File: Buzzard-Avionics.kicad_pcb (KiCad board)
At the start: 2 copper layers, 30 x 115.5 mm, 6 parts, among them J4 Conn_01x02_Socket, SW1 SW_SPDT

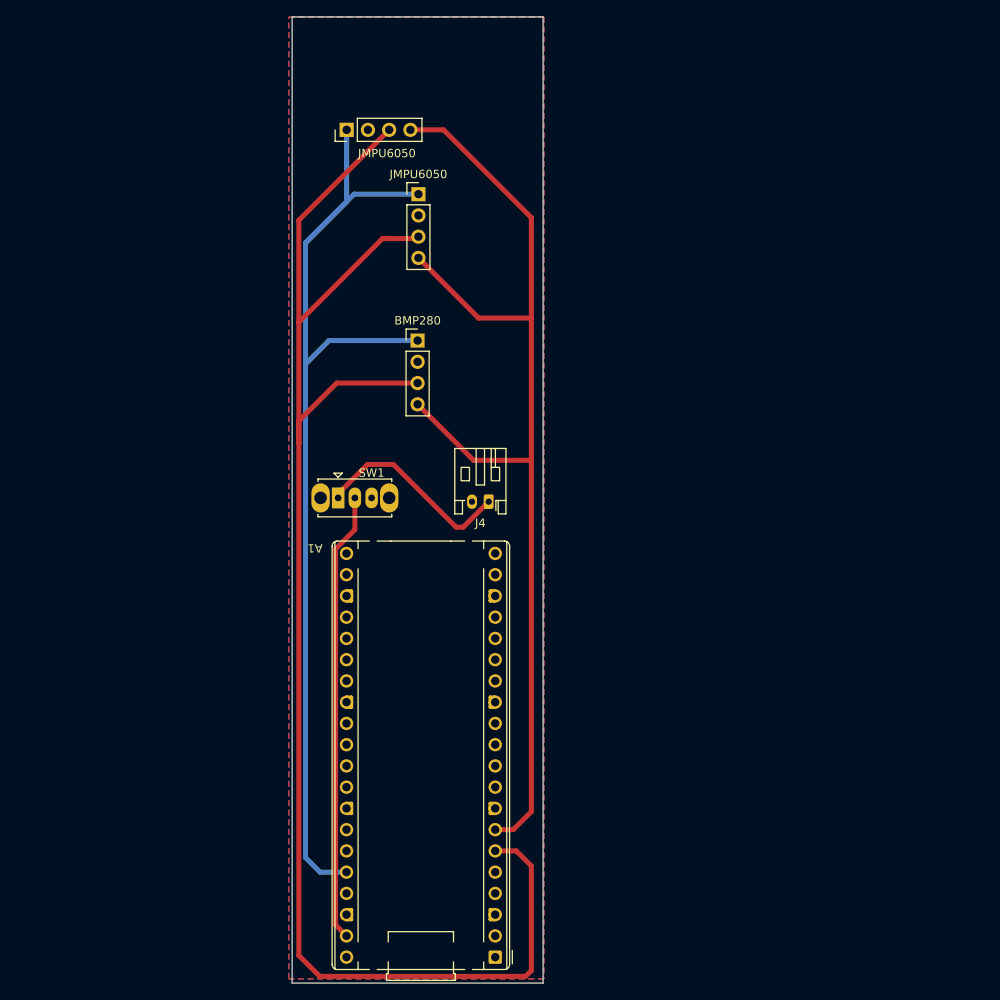
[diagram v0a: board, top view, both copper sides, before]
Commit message: Releases/Mayor added
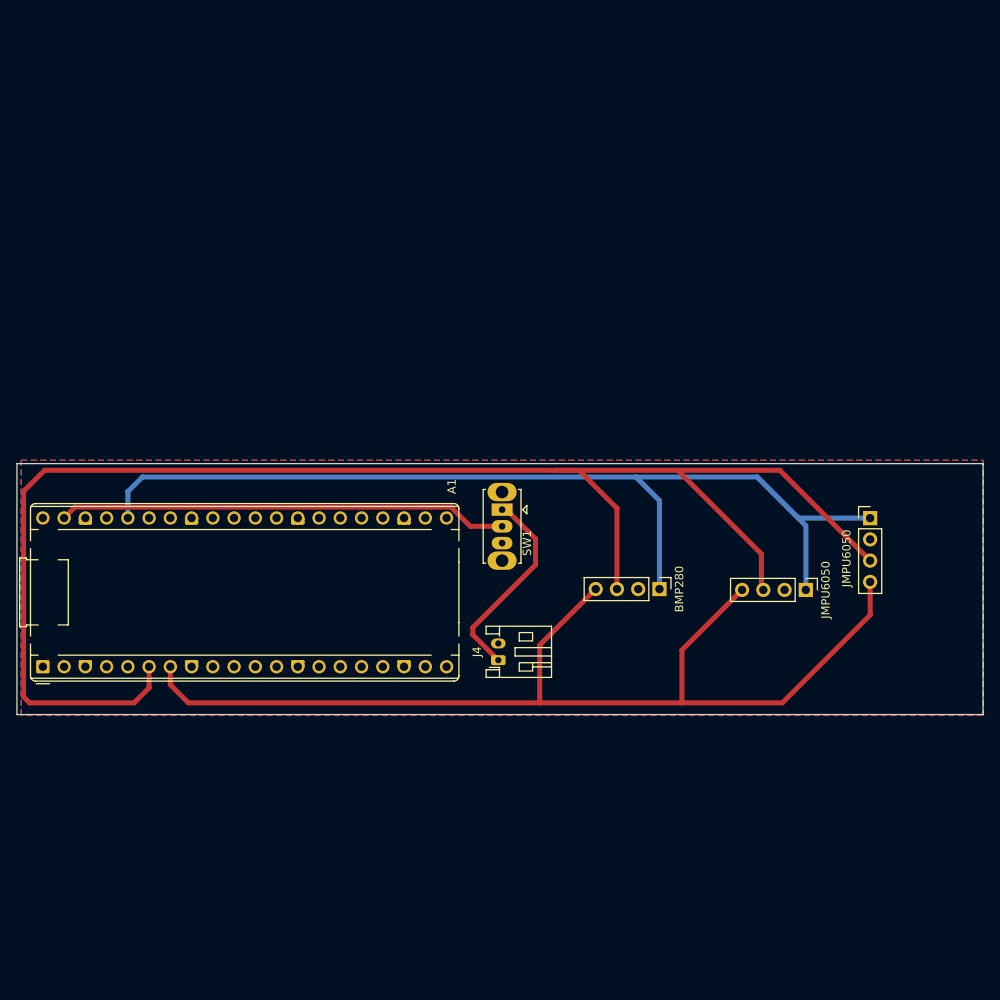
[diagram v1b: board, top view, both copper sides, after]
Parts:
- moved JMPU6050 77.9 mm to (196.5, 115.9), turned to 0 degrees
- moved JMPU6050 66.2 mm to (188.8, 124.5), turned to -90 degrees
- moved A1 64.3 mm to (97.6, 133.7), turned to 90 degrees
- moved BMP280 41.5 mm to (171.3, 124.4), turned to -90 degrees
- moved SW1 19.6 mm to (152.5, 114.9), turned to -90 degrees
- moved J4 19.0 mm to (152.1, 132.9), turned to 90 degrees
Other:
- board size 30 x 115.5 mm -> 115.5 x 30 mm
